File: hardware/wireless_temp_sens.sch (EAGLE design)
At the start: 32 parts, among them Q1 BC550C, Q2 32.768kHz, Q3 1MHz

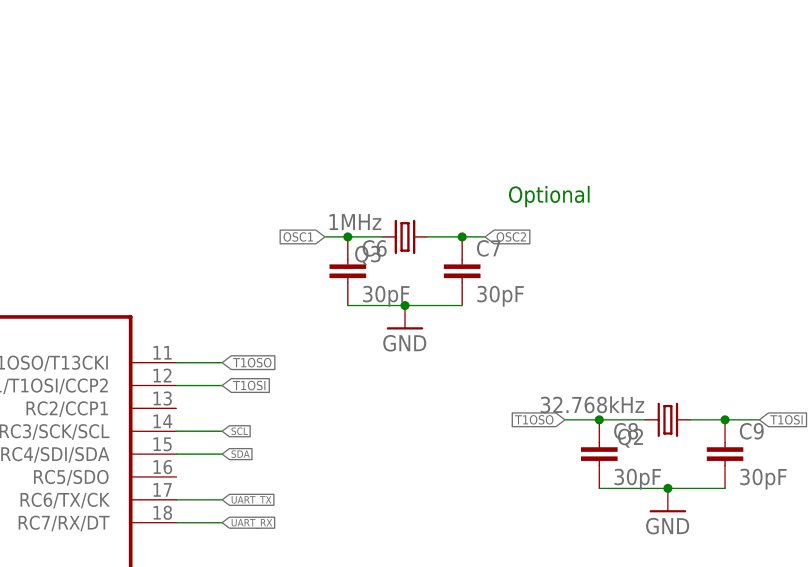
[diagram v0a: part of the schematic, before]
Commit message: update board schema
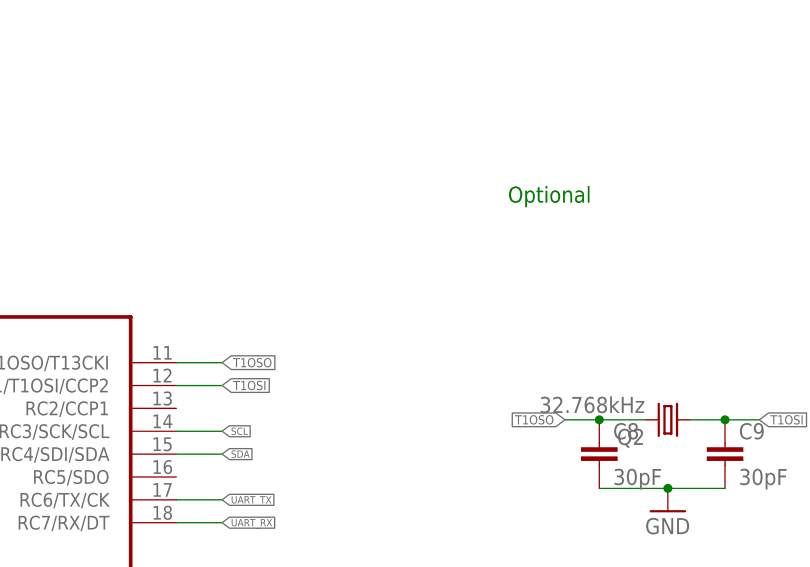
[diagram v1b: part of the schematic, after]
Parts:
- removed C6, C7: 30pF, rcl:C-EU025-024X044
- removed Q3: 1MHz, crystal:CRYSTALHC49S
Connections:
- net GND: no longer C6.2, C7.2
- net OSC1: no longer C6.1, Q3.2
- net OSC2: no longer C7.1, Q3.1
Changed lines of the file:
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@@
 <setting verticaltext="up"/>
 </settings>
-<grid distance="0.05" unitdist="inch" unit="inch" style="dots" multiple="1" display="yes" altdistance="0.025" altunitdist="inch" altunit="inch"/>
+<grid distance="0.1" unitdist="inch" unit="inch" style="lines" multiple="1" display="no" altdistance="0.01" altunitdist="inch" altunit="inch"/>
 <layers>
 <layer number="1" name="Top" color="4" fill="1" visible="no" active="no"/>
@@
 </classes>
 <parts>
-<part name="FRAME1" library="frames" deviceset="DINA4_L" device="" value="XBee Temp Hyd. sensor"/>
+<part name="WIRELESS_SENSOR" library="frames" deviceset="DINA4_L" device="" value="XBee Temp Hyd. sensor"/>
 <part name="SUPPLY" library="ma_libs" deviceset="3AA" device=""/>
 <part name="UC1" library="ma_libs" deviceset="S7V8" device=""/>
@@
 <part name="GND14" library="supply1" deviceset="GND" device=""/>
 <part name="Q2" library="crystal" deviceset="CRYSTAL" device="TC26H" value="32.768kHz"/>
-<part name="Q3" library="crystal" deviceset="CRYSTAL" device="HC49S" value="1MHz"/>
-<part name="GND15" library="supply1" deviceset="GND" device=""/>
-<part name="C6" library="rcl" deviceset="C-EU" device="025-024X044" value="30pF"/>
-<part name="C7" library="rcl" deviceset="C-EU" device="025-024X044" value="30pF"/>
 <part name="C8" library="rcl" deviceset="C-EU" device="025-024X044" value="30pF"/>
 <part name="C9" library="rcl" deviceset="C-EU" device="025-024X044" value="30pF"/>
@@
 </plain>
 <instances>
-<instance part="FRAME1" gate="G$1" x="0" y="0"/>
-<instance part="FRAME1" gate="G$2" x="162.56" y="0"/>
+<instance part="WIRELESS_SENSOR" gate="G$1" x="0" y="0"/>
+<instance part="WIRELESS_SENSOR" gate="G$2" x="162.56" y="0"/>
 <instance part="SUPPLY" gate="G$1" x="7.62" y="152.4" rot="R270"/>
 <instance part="UC1" gate="G$1" x="38.1" y="149.86"/>
@@
 <instance part="GND14" gate="1" x="246.38" y="45.72"/>
 <instance part="Q2" gate="G$1" x="242.57" y="125.73" rot="R180"/>
-<instance part="Q3" gate="G$1" x="213.36" y="146.05" rot="R180"/>
-<instance part="GND15" gate="1" x="213.36" y="135.89"/>
-<instance part="C6" gate="G$1" x="207.01" y="143.51"/>
-<instance part="C7" gate="G$1" x="219.71" y="143.51"/>
 <instance part="C8" gate="G$1" x="234.95" y="123.19"/>
 <instance part="C9" gate="G$1" x="248.92" y="123.19"/>
@@
 </segment>
 <segment>
-<pinref part="C6" gate="G$1" pin="2"/>
-<pinref part="GND15" gate="1" pin="GND"/>
-<wire x1="207.01" y1="138.43" x2="213.36" y2="138.43" width="0.1524" layer="91"/>
-<pinref part="C7" gate="G$1" pin="2"/>
-<wire x1="219.71" y1="138.43" x2="213.36" y2="138.43" width="0.1524" layer="91"/>
-<junction x="213.36" y="138.43"/>
-</segment>
-<segment>
 <pinref part="C8" gate="G$1" pin="2"/>
 <pinref part="GND16" gate="1" pin="GND"/>
@@
 <label x="63.5" y="106.68" size="1.016" layer="95" rot="R180" xref="yes"/>
 </segment>
-<segment>
-<pinref part="Q3" gate="G$1" pin="1"/>
-<pinref part="C7" gate="G$1" pin="1"/>
-<wire x1="215.9" y1="146.05" x2="219.71" y2="146.05" width="0.1524" layer="91"/>
-<wire x1="219.71" y1="146.05" x2="222.25" y2="146.05" width="0.1524" layer="91"/>
-<junction x="219.71" y="146.05"/>
-<label x="222.25" y="146.05" size="1.016" layer="95" xref="yes"/>
-</segment>
 </net>
 <net name="OSC1" class="0">
@@
 <label x="63.5" y="104.14" size="1.016" layer="95" rot="R180" xref="yes"/>
 </segment>
-<segment>
-<pinref part="C6" gate="G$1" pin="1"/>
-<pinref part="Q3" gate="G$1" pin="2"/>
-<wire x1="207.01" y1="146.05" x2="210.82" y2="146.05" width="0.1524" layer="91"/>
-<wire x1="207.01" y1="146.05" x2="204.47" y2="146.05" width="0.1524" layer="91"/>
-<junction x="207.01" y="146.05"/>
-<label x="204.47" y="146.05" size="1.016" layer="95" rot="R180" xref="yes"/>
-</segment>
-</net>
+</net>
